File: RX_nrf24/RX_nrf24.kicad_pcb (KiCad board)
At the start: 2 copper layers, 50 x 25 mm, 54 parts, among them J1 USB_B_Micro, J2 Conn_01x03_Male, J3 Conn_Coaxial, J4 Conn_01x10_Male, J5 Conn_01x04_Female, SW1 SW_Push, U1 USBLC6-2SC6, U2 AMS1117-3.3, U3 STM32F103C8Tx, U4 RFX2401C, U5 nRF24L01P, Y1 Crystal_GND24, Y2 Crystal_GND24

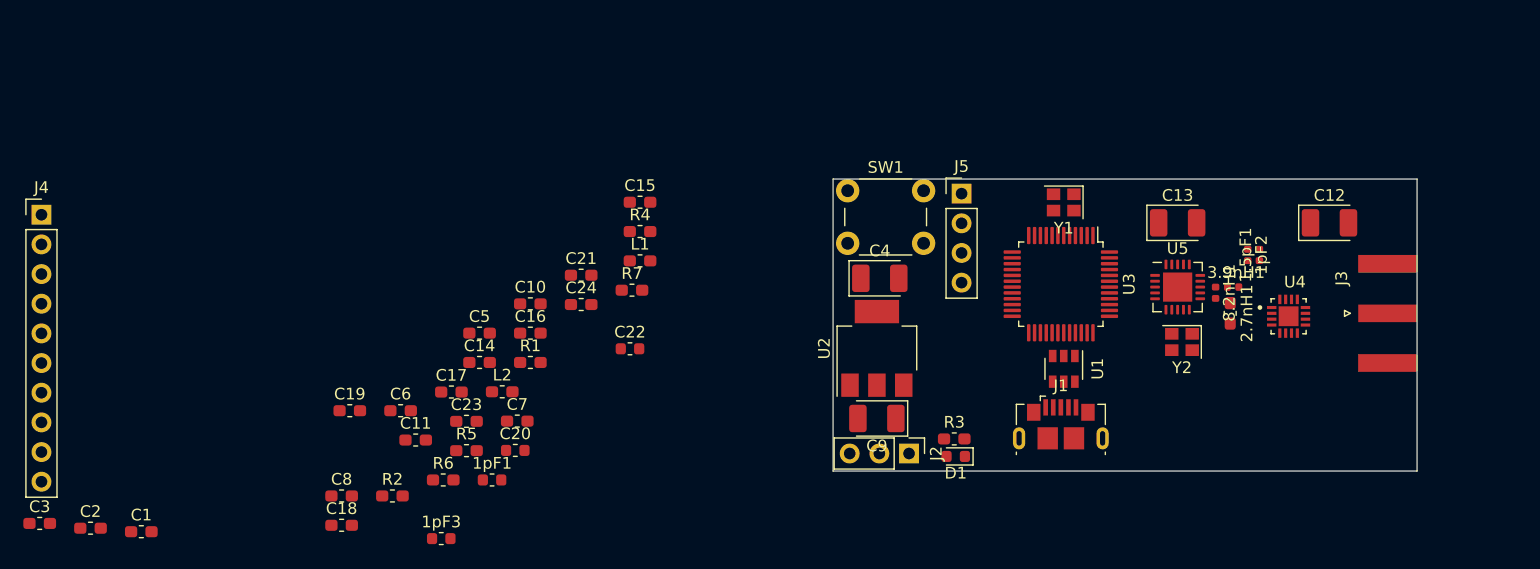
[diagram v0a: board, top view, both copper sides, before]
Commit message: a
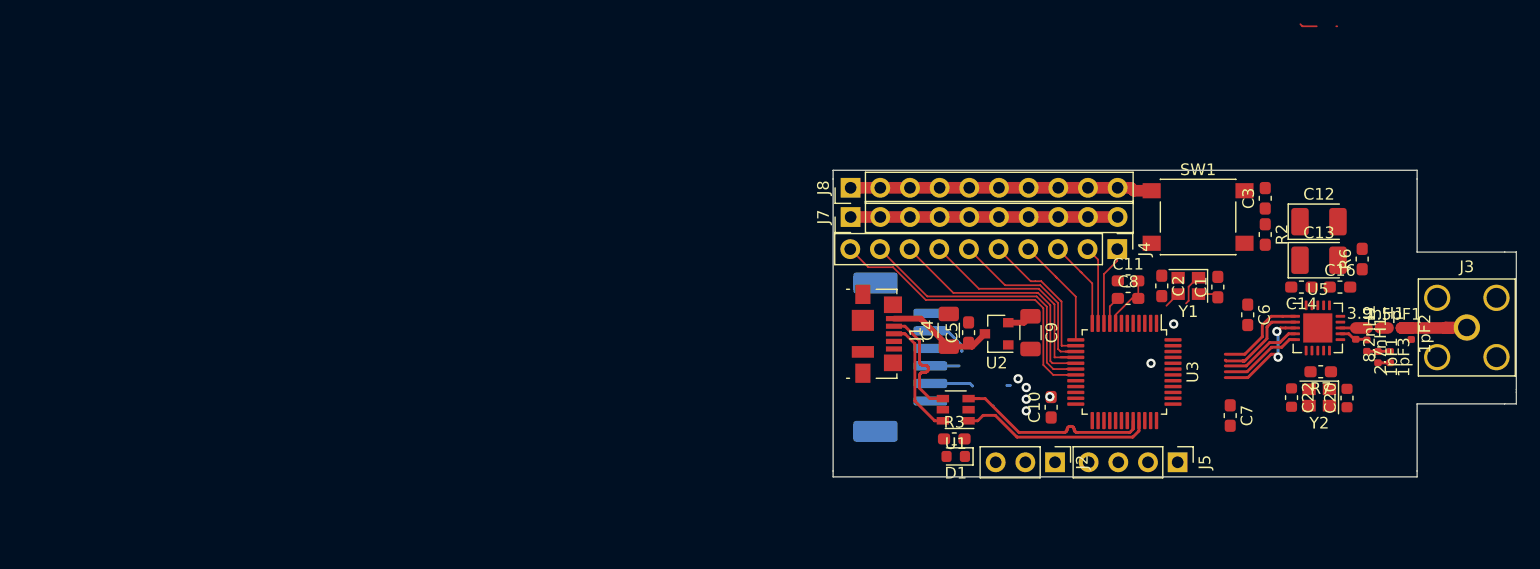
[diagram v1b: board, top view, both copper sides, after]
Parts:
- removed C15, C17, C18, C19, C21, C23, C24: C, Capacitor_SMD:C_0603_1608Metric_Pad1.05x0.95mm_HandSolder
- removed L1, L2: L, Capacitor_SMD:C_0603_1608Metric_Pad1.05x0.95mm_HandSolder
- removed R1: 1M, Resistor_SMD:R_0603_1608Metric_Pad1.05x0.95mm_HandSolder
- removed R4, R5: R, Resistor_SMD:R_0603_1608Metric_Pad1.05x0.95mm_HandSolder
- removed U4: RFX2401C, RF:QFN50P300X300X60-17N
- added J6: Conn_01x06_Male, Connector_JST:JST_ZE_SM06B-ZESS-TB_1x06-1MP_P1.50mm_Horizontal, B.Cu at (155.8, 102.5)
- added J7: Conn_01x10_Male, Connector_PinHeader_2.54mm:PinHeader_1x10_P2.54mm_Vertical, F.Cu at (151.5, 90.5)
- added J8: Conn_01x10_Male, Connector_PinHeader_2.54mm:PinHeader_1x10_P2.54mm_Vertical, F.Cu at (151.5, 88.0)
- 1pF1, 1pF3: footprint Capacitor_SMD:C_0603_1608Metric -> Capacitor_SMD:C_0402_1005Metric
- 2.7nH1: footprint Capacitor_SMD:C_0603_1608Metric_Pad1.05x0.95mm_HandSolder -> Capacitor_SMD:C_0402_1005Metric
- C4, C9: footprint Capacitor_Tantalum_SMD:CP_EIA-3528-12_Kemet-T_Pad1.50x2.35mm_HandSolder -> Capacitor_SMD:C_1206_3216Metric
- J1: footprint Connector_USB:USB_Micro-B_GCT_USB3076-30-A -> Connector_USB:USB_Micro-B_Molex_47346-0001
- J3: footprint Connector_Coaxial:SMA_Amphenol_132289_EdgeMount -> Connector_Coaxial:SMA_Amphenol_132203-12_Horizontal
- SW1: footprint Button_Switch_THT:SW_PUSH_6mm_H5mm -> Button_Switch_SMD:SW_Push_1P1T_NO_6x6mm_H9.5mm
- U2: value AMS1117-3.3 -> MCP1700-3302E_SOT23; footprint Package_TO_SOT_SMD:SOT-223-3_TabPin2 -> Package_TO_SOT_SMD:SOT-23
- moved C3 108.6 mm to (187.0, 88.9), turned to 90 degrees
- moved C1 94.5 mm to (182.9, 96.5), turned to 90 degrees
- moved C2 94.0 mm to (178.1, 96.4), turned to 270 degrees
- moved J4 92.2 mm to (174.3, 93.2), turned to 270 degrees
- moved 1pF3 82.7 mm to (197.7, 102.5), turned to 270 degrees
- moved R6 80.9 mm to (195.3, 94.1), turned to 90 degrees
- moved R2 78.0 mm to (187.0, 92.0), turned to 270 degrees
- moved 1pF1 76.6 mm to (196.7, 102.5), turned to 270 degrees
- moved C6 73.0 mm to (185.5, 98.9), turned to 270 degrees
- moved C20 71.4 mm to (194.0, 106.0), turned to 90 degrees
- moved C14 70.7 mm to (190.1, 96.5), turned to 180 degrees
- moved C16 69.4 mm to (193.4, 96.5)
- moved C8 69.4 mm to (175.3, 97.5)
- moved C11 62.5 mm to (175.3, 96.0)
- moved C7 61.0 mm to (184.0, 107.5), turned to 270 degrees
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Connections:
- J3 pad 1: Net-(C23-Pad1) -> RF_out
- U3 pad 10: Net-(U3-Pad10) -> P1
- U3 pad 11: Net-(U3-Pad11) -> P2
- U3 pad 12: Net-(U3-Pad12) -> P3
- U3 pad 13: Net-(U3-Pad13) -> P4
- U3 pad 14: Net-(U3-Pad14) -> P5
- U3 pad 15: Net-(U3-Pad15) -> P6
- U3 pad 16: Net-(U3-Pad16) -> P7
- U3 pad 17: Net-(U3-Pad17) -> P8
- U3 pad 18: Net-(U3-Pad18) -> P9
- U3 pad 19: Net-(U3-Pad19) -> P10
- U3 pad 21: Net-(U3-Pad21) -> UART3_TX
- U3 pad 22: Net-(U3-Pad22) -> UART3_RX
- U3 pad 26: Net-(U3-Pad26) -> UART3_CTS
- U3 pad 27: Net-(U3-Pad27) -> UART3_RTS
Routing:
- net GND: track 0.00 -> 31.7 mm, vias 0 -> 1
- net +3V3: track 0.00 -> 27.4 mm
- net P10: track 0.00 -> 27.4 mm
- net P9: track 0.00 -> 24.6 mm
- net P8: track 0.00 -> 21.9 mm
- net P7: track 0.00 -> 19.5 mm
- net USB_D-: track 0.00 -> 17.5 mm
- net USB_D+: track 0.00 -> 16.8 mm
- net P6: track 0.00 -> 16.0 mm
- net P5: track 0.00 -> 12.2 mm
- net D+: track 0.00 -> 10.9 mm
- net D-: track 0.00 -> 10.1 mm
- net SCK: track 0.00 -> 9.79 mm, vias 0 -> 2
- net P4: track 0.00 -> 9.60 mm
- net +5V: track 0.00 -> 9.24 mm
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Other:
- board size 50 x 25 mm -> 58.5 x 26.2 mm
- net class Default: clearance 0.2 -> 0.15
- rule trace_clearance: 0.2 -> 0.15
- rule trace_min: 0.2 -> 0.15
